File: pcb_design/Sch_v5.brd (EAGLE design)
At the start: 93 x 53 mm, 30 parts

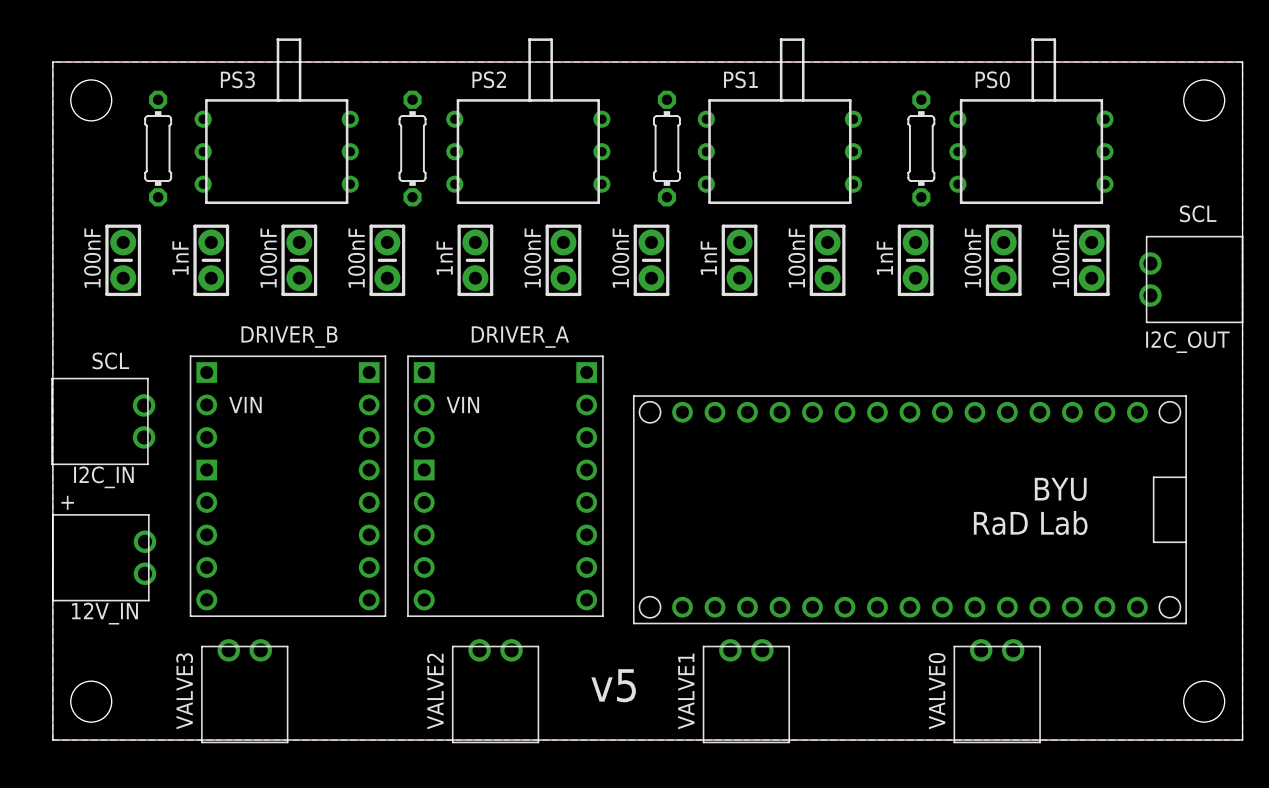
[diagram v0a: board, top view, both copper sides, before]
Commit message: board routed
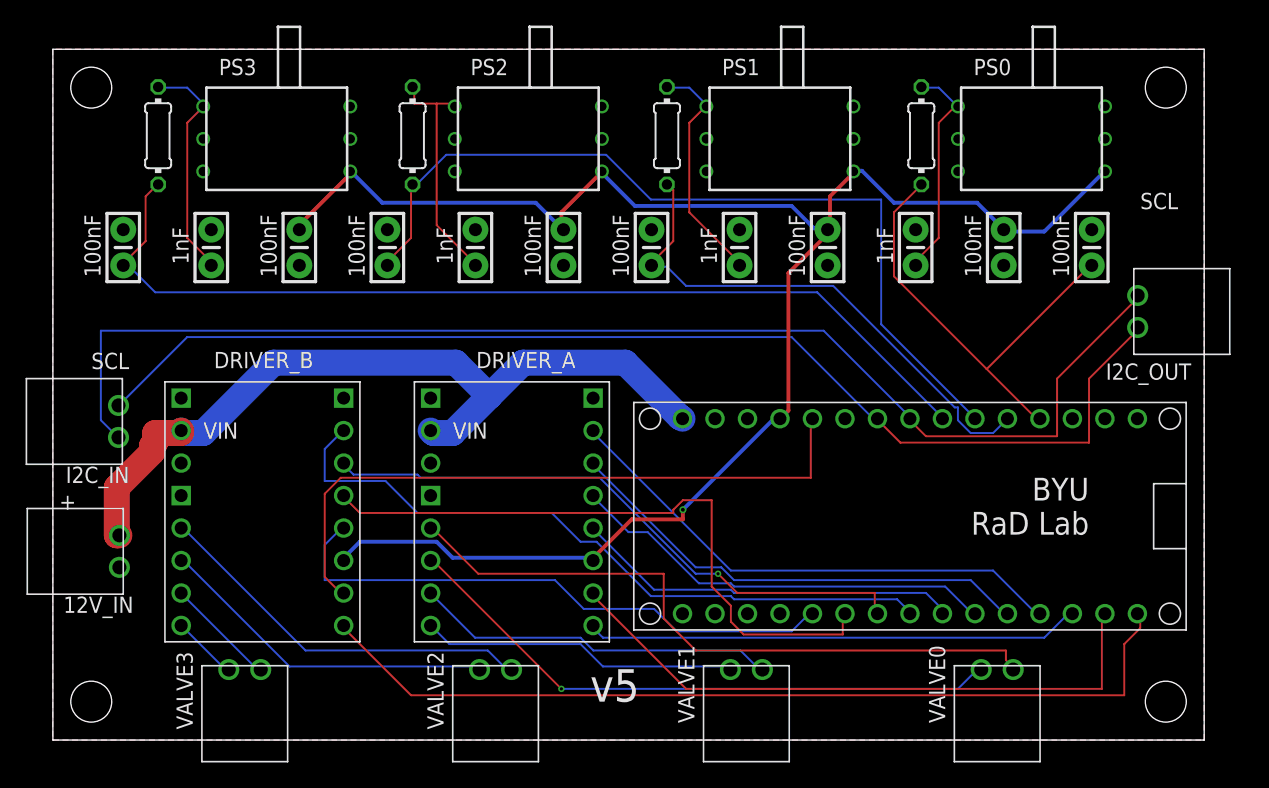
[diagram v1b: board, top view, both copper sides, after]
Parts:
- moved DRIVER_B 2.83 mm to (24.0, 28.0)
- moved I2C_OUT 2.69 mm to (92.0, 33.5)
- moved 12V_IN 2.06 mm to (-2.00, 14.8)
- moved DRIVER_A 2.06 mm to (43.5, 28.0)
- moved I2C_IN 2.00 mm to (-2.07, 24.9)
- moved VALVE0 1.50 mm to (73.8, -1.69)
- moved VALVE1 1.50 mm to (54.2, -1.69)
- moved VALVE2 1.50 mm to (34.6, -1.69)
- moved VALVE3 1.50 mm to (15.0, -1.69)
- moved C1 1.00 mm to (67.4, 38.5)
- moved C10 1.00 mm to (46.8, 38.5)
- moved C11 1.00 mm to (26.1, 38.5)
- moved C12 1.00 mm to (5.50, 38.5)
- moved C2 1.00 mm to (53.7, 38.5)
- moved C3 1.00 mm to (33.0, 38.5)
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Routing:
- net 5V: track 0.00 -> 136.3 mm, vias 0 -> 1
- net SDA: track 0.00 -> 100.9 mm
- net SCL: track 0.00 -> 92.1 mm
- net A3: track 0.00 -> 76.6 mm
- net EF1_B: track 0.00 -> 70.4 mm
- net A2: track 0.00 -> 66.3 mm
- net 12V: track 0.00 -> 63.0 mm
- net D5: track 0.00 -> 54.7 mm
- net N$8: track 0.00 -> 52.7 mm
- net EF2_B: track 0.00 -> 51.7 mm
- net D3: track 0.00 -> 50.9 mm
- net EF2_A: track 0.00 -> 49.0 mm
- net N$7: track 0.00 -> 47.8 mm, vias 0 -> 1
- net D4: track 0.00 -> 47.5 mm, vias 0 -> 1
- net D2: track 0.00 -> 45.1 mm
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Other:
- board size 93 x 53 mm -> 90 x 54 mm
